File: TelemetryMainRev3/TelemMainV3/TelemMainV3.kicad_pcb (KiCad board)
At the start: 2 copper layers, 187.9 x 88.1 mm, 38 parts, among them J1 8 pin ATM connector, J3 12 pin ATM connector, J4 SD to SPI (Molex nanofit), J5 F3311A7H121030E200, U1 LM7805_TO220, U2 LM7809_TO220, U3 NUCLEO-F446RE, U4 ISO1050DUB, U5 XBP9B-DPST-001, U6 MCP6004

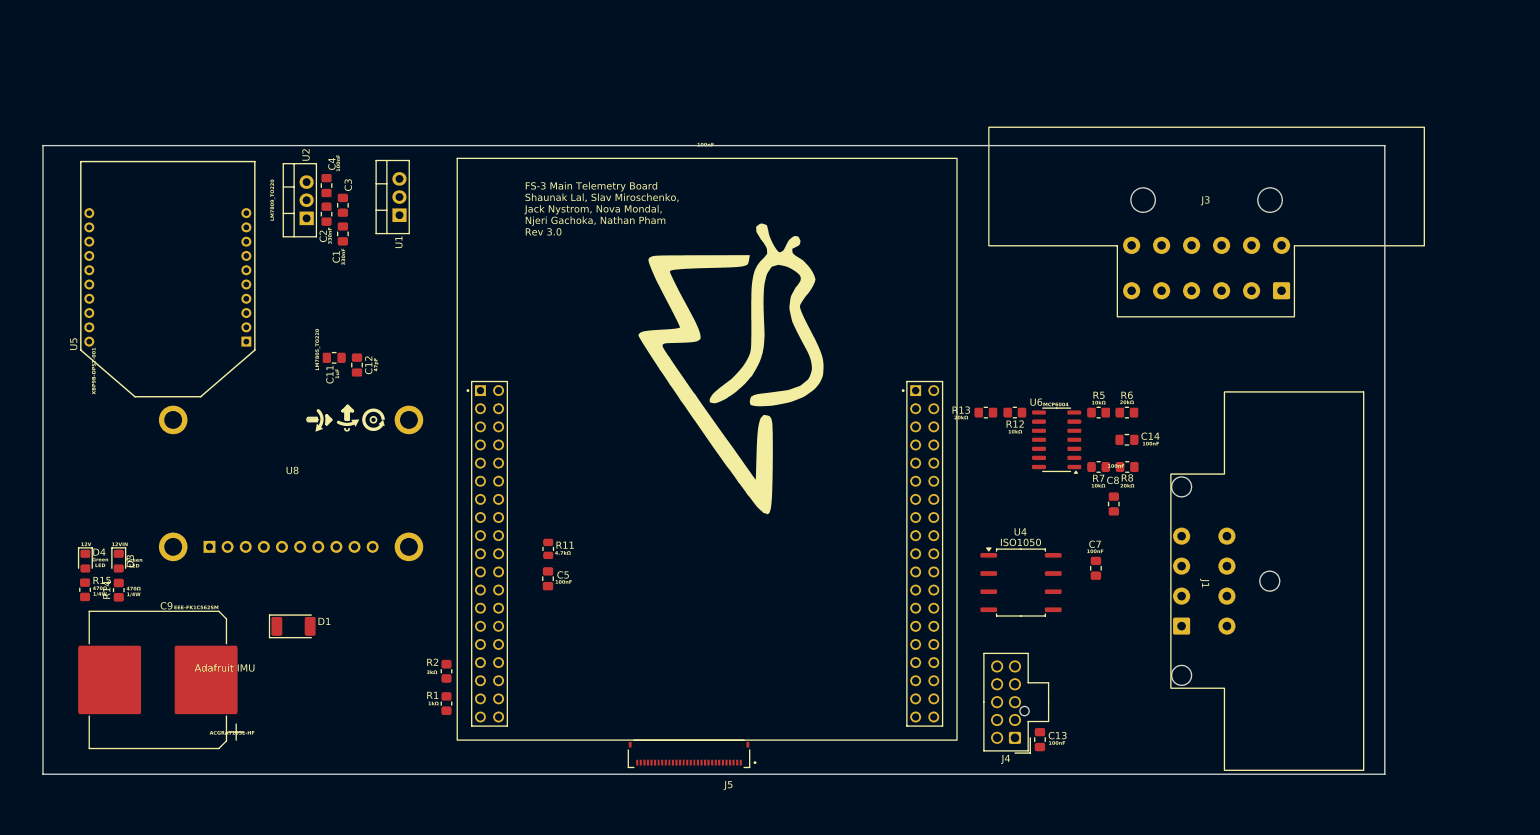
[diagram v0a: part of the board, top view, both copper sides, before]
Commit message: Telemetry Main Rev 3 finished
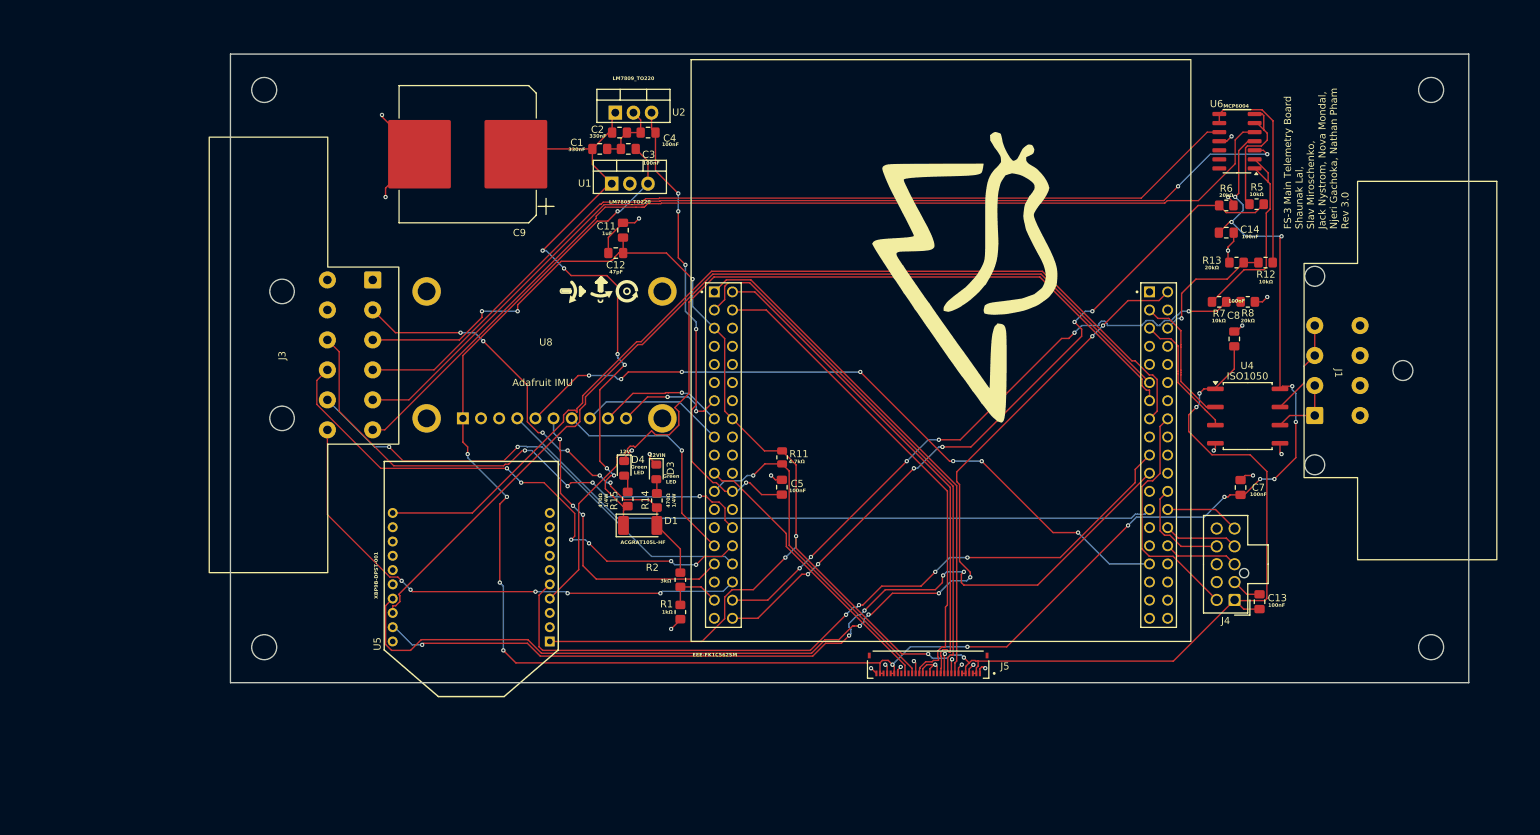
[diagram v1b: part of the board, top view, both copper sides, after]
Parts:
- added REF**: MountingHole_3.5mm, MountingHole:MountingHole_3.5mm, F.Cu at (228.9, 57.0)
- added REF**: MountingHole_3.5mm, MountingHole:MountingHole_3.5mm, F.Cu at (65.5, 135.1)
- added REF**: MountingHole_3.5mm, MountingHole:MountingHole_3.5mm, F.Cu at (228.9, 135.1)
- added REF**: MountingHole_3.5mm, MountingHole:MountingHole_3.5mm, F.Cu at (65.5, 57.0)
- moved J3 121.6 mm to (64.3, 114.6), turned to 90 degrees
- moved C9 85.5 mm to (94.0, 66.0)
- moved R15 77.1 mm to (116.4, 114.3)
- moved D4 76.6 mm to (115.9, 110.0)
- moved R14 76.4 mm to (120.5, 114.5)
- moved D3 76.3 mm to (120.4, 110.5)
- moved U5 59.8 mm to (94.5, 125.5)
- moved D1 50.6 mm to (118.2, 118.0)
- moved U6 48.9 mm to (201.8, 64.2)
- moved U2 45.7 mm to (114.7, 60.2), turned to 0 degrees
- moved C4 45.6 mm to (119.3, 63.0), turned to 180 degrees
- moved C11 44.2 mm to (115.8, 76.6), turned to 90 degrees
- moved C2 42.6 mm to (115.3, 63.0), turned to 0 degrees
- moved R12 40.9 mm to (205.8, 81.2)
- moved R13 40.9 mm to (201.7, 81.2)
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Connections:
- J5 pad 2: +3.3V -> +3V3
- J5 pad 3: +3.3V -> +3V3
- J5 pad 5: +3.3V -> +3V3
- J5 pad 6: +3.3V -> +3V3
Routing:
- net +3V3: track 0.00 -> 275.0 mm, vias 0 -> 9
- net +5V: track 0.00 -> 271.7 mm, vias 0 -> 16
- net Radio CS1: track 0.00 -> 150.6 mm, vias 0 -> 6
- net Brake Sensor B: track 0.00 -> 143.0 mm
- net Brake Sensor F: track 0.00 -> 141.5 mm, vias 0 -> 2
- net Radio MOSI1: track 0.00 -> 135.0 mm
- net Radio SCK1: track 0.00 -> 134.9 mm
- net Steering Sensor: track 0.00 -> 132.4 mm
- net Radio MISO1: track 0.00 -> 127.9 mm
- net Radio ATTN: track 0.00 -> 123.1 mm, vias 0 -> 5
- net Radio Reset: track 0.00 -> 107.5 mm, vias 0 -> 4
- net Brake Sensor R 3V3: track 0.00 -> 101.9 mm, vias 0 -> 6
- net IMU SDA: track 0.00 -> 100.3 mm, vias 0 -> 7
- net IMU SCL: track 0.00 -> 94.9 mm
- net Brake Sensor F 3V3: track 0.00 -> 90.0 mm, vias 0 -> 6
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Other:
- board size 187.9 x 88.1 mm -> 173.4 x 88.1 mm
